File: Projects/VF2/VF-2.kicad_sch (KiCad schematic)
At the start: 16 parts, among them U1 OPA2134, U3 OPA2134

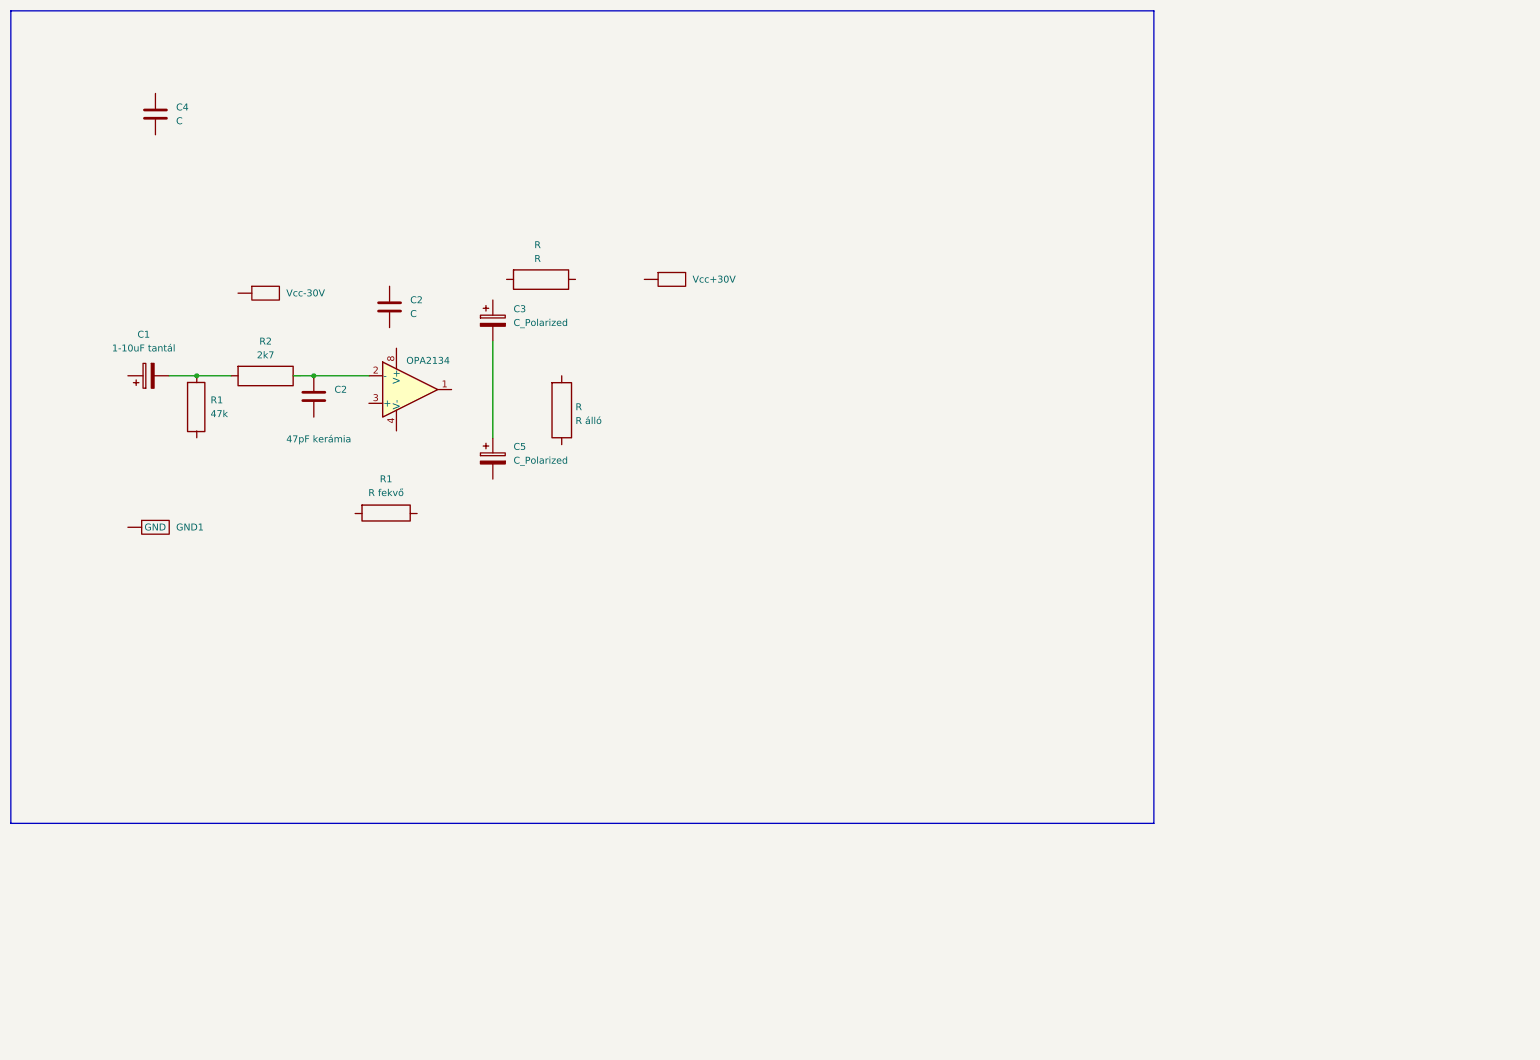
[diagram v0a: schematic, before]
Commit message: 1
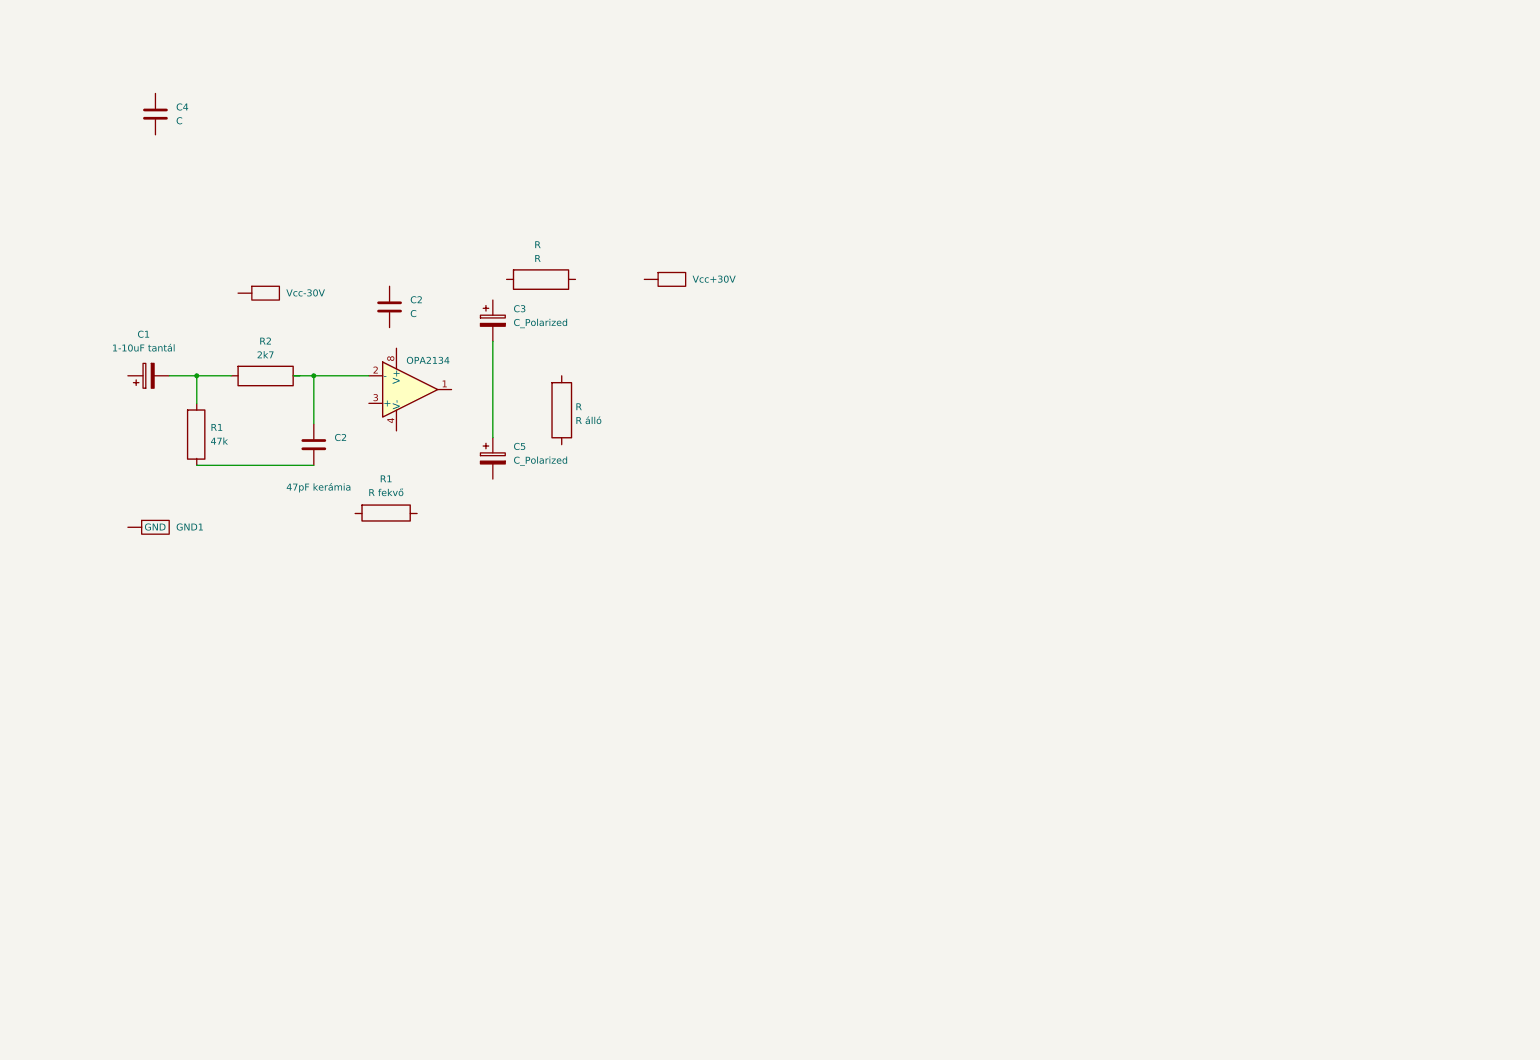
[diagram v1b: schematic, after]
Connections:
- net at C2.2: now also R1.1
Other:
- moved on the sheet: C2, R1
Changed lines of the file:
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@@
 	(generator_version "10.0")
 	(paper "A4")
-	(text_box ""
-		(exclude_from_sim no)
-		(at 0 0 0)
-		(size 210.82 149.86)
-		(margins 0.9525 0.9525 0.9525 0.9525)
-		(stroke
-			(width 0)
-			(type solid)
-		)
-		(fill
-			(type none)
-		)
-		(effects
-			(font
-				(size 1.27 1.27)
-			)
-			(justify left top)
-		)
+	(junction
+		(at 34.29 67.31)
+		(diameter 0)
+		(color 0 0 0 0)
 	)
 	(junction
@@
 		(color 0 0 0 0)
 	)
-	(junction
-		(at 34.29 67.31)
-		(diameter 0)
-		(color 0 0 0 0)
-	)
 	(wire
 		(pts
@@
 	(wire
 		(pts
-			(xy 29.21 67.31) (xy 34.29 67.31)
+			(xy 34.29 67.31) (xy 40.64 67.31)
 		)
 		(stroke
@@
 	(wire
 		(pts
-			(xy 66.04 67.31) (xy 55.88 67.31)
+			(xy 55.88 67.31) (xy 55.88 76.2)
 		)
 		(stroke
@@
 	(wire
 		(pts
-			(xy 88.9 60.96) (xy 88.9 78.74)
+			(xy 29.21 67.31) (xy 34.29 67.31)
 		)
 		(stroke
@@
 	(wire
 		(pts
-			(xy 34.29 67.31) (xy 40.64 67.31)
+			(xy 88.9 60.96) (xy 88.9 78.74)
 		)
 		(stroke
@@
 		)
 	)
+	(wire
+		(pts
+			(xy 34.29 72.39) (xy 34.29 67.31)
+		)
+		(stroke
+			(width 0)
+			(type default)
+		)
+	)
+	(wire
+		(pts
+			(xy 55.88 67.31) (xy 66.04 67.31)
+		)
+		(stroke
+			(width 0)
+			(type default)
+		)
+	)
+	(wire
+		(pts
+			(xy 34.29 83.82) (xy 55.88 83.82)
+		)
+		(stroke
+			(width 0)
+			(type default)
+		)
+	)
 	(symbol
 		(lib_id "Device:C")
@@
 	(symbol
 		(lib_id "Device:C")
-		(at 55.88 71.12 0)
+		(at 55.88 80.01 0)
 		(unit 1)
 		(body_style 1)
@@
 		(dnp no)
 		(property "Reference" "C2"
-			(at 59.69 69.8499 0)
+			(at 59.69 78.7399 0)
 			(show_name no)
 			(do_not_autoplace no)
@@
 		)
 		(property "Value" "47pF kerámia"
-			(at 50.8 78.994 0)
+			(at 50.8 87.884 0)
 			(show_name no)
 			(do_not_autoplace no)
@@
 		)
 		(property "Footprint" "Package_SO:SOIC-8_3.9x4.9mm_P1.27mm"
-			(at 56.8452 74.93 0)
-			(hide yes)
-			(show_name no)
-			(do_not_autoplace no)
-			(effects
-				(font
-					(size 1.27 1.27)
-				)
-			)
-		)
-		(property "Datasheet" ""
-			(at 55.88 71.12 0)
+			(at 56.8452 83.82 0)
+			(hide yes)
+			(show_name no)
+			(do_not_autoplace no)
+			(effects
+				(font
+					(size 1.27 1.27)
+				)
+			)
+		)
+		(property "Datasheet" ""
+			(at 55.88 80.01 0)
 			(hide yes)
 			(show_name no)
@@
 		)
 		(property "Description" "Unpolarized capacitor"
-			(at 55.88 71.12 0)
+			(at 55.88 80.01 0)
 			(hide yes)
 			(show_name no)
@@
 		(lib_name "R_álló_1")
 		(lib_id "001_Resistor_user:R_álló")
-		(at 34.29 76.2 0)
+		(at 34.29 81.28 0)
 		(unit 1)
 		(body_style 1)
@@
 		(fields_autoplaced yes)
 		(property "Reference" "R1"
-			(at 36.83 71.7998 0)
+			(at 36.83 76.8798 0)
 			(show_name no)
 			(do_not_autoplace no)
@@
 		)
 		(property "Value" "47k"
-			(at 36.83 74.3398 0)
+			(at 36.83 79.4198 0)
 			(show_name no)
 			(do_not_autoplace no)
@@
 		)
 		(property "Footprint" ""
-			(at 32.512 76.2 90)
-			(hide yes)
-			(show_name no)
-			(do_not_autoplace no)
-			(effects
-				(font
-					(size 1.27 1.27)
-				)
-			)
-		)
-		(property "Datasheet" ""
-			(at 34.29 76.2 0)
+			(at 32.512 81.28 90)
+			(hide yes)
+			(show_name no)
+			(do_not_autoplace no)
+			(effects
+				(font
+					(size 1.27 1.27)
+				)
+			)
+		)
+		(property "Datasheet" ""
+			(at 34.29 81.28 0)
 			(hide yes)
 			(show_name no)
@@
 		)
 		(property "Description" "Resistor"
-			(at 36.195 70.485 90)
-			(hide yes)
-			(show_name no)
+			(at 36.195 75.565 90)
+			(hide yes)
+			(show_name no)

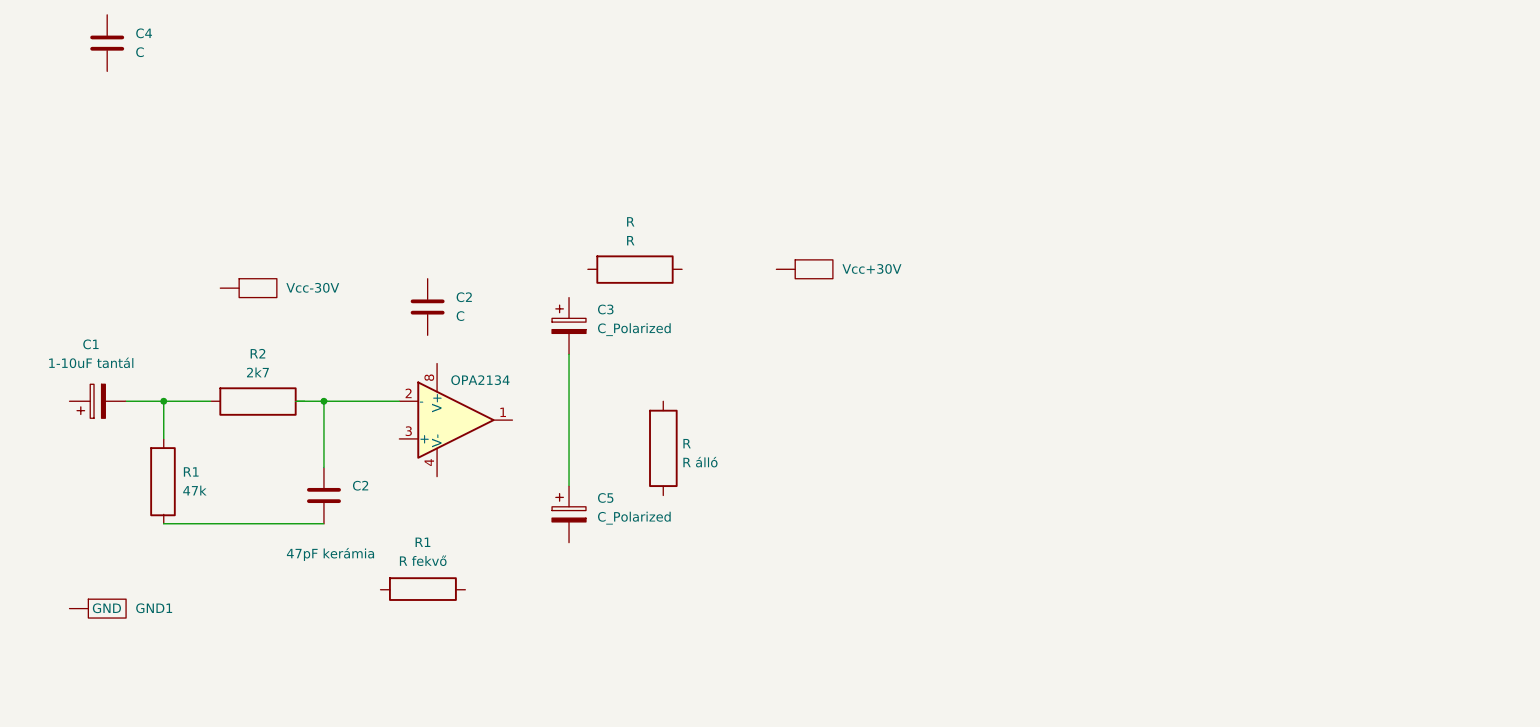
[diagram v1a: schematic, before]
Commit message: sch
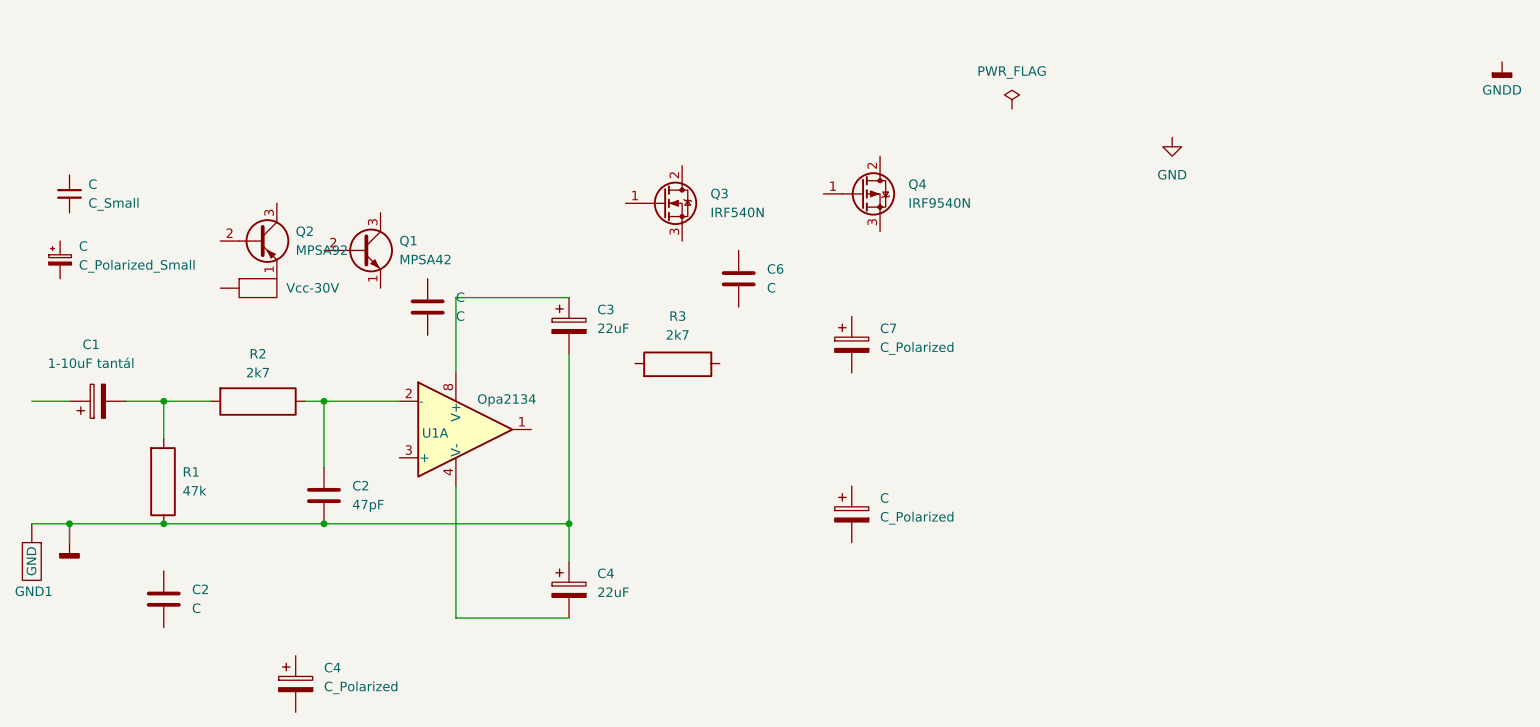
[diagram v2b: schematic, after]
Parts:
- removed C4: C, Package_SO:SOIC-8_3.9x4.9mm_P1.27mm, symbol Device:C
- removed R: R, symbol 001_Resistor_user:R
- removed R: R álló, symbol 001_Resistor_user:R_álló
- removed R1: R fekvő, symbol 001_Resistor_user:R
- removed U1: OPA2134, symbol Amplifier_Operational:OPA2134
- removed Vcc+30V: (no value), symbol 000_Device:Vcc
- added C: C_Polarized_Small, Package_SO:SOIC-8_3.9x4.9mm_P1.27mm, symbol Device:C_Polarized_Small
- added C: C_Small, symbol Device:C_Small
- added C, C4, C7: C_Polarized, Package_SO:SOIC-8_3.9x4.9mm_P1.27mm, symbol 000_Device:C_Polarized
- added C2, C6: C, Package_SO:SOIC-8_3.9x4.9mm_P1.27mm, symbol 000_Device:C
- added Q1: MPSA42, Package_TO_SOT_THT:TO-92_Inline, symbol Transistor_BJT:MPSA42
- added Q2: MPSA92, Package_TO_SOT_THT:TO-92_Inline, symbol Transistor_BJT:MPSA92
- added Q3: IRF540N, Package_TO_SOT_THT:TO-220-3_Vertical, symbol Transistor_FET:IRF540N
- added Q4: IRF9540N, Package_TO_SOT_THT:TO-220-3_Vertical, symbol Transistor_FET:IRF9540N
- added R3: 2k7, Package_SO:SOIC-8_3.9x4.9mm_P1.27mm, symbol 000_Device:R
- added U4: OPA2134, symbol 000_Device:OPA2134
- C2: value 47pF kerámia -> 47pF
- C3: value C_Polarized -> 22uF
- C4: renamed from C5; value C_Polarized -> 22uF
- U1: renamed from U3; value OPA2134 -> Opa2134
- renumbered C2 to C
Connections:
- net at R2.2: now also C2.1, U1.2 (-)
- net at C3.2, C4.1: now also C2.2, GND1. (GND), R1.1
- net at C4.2: now also U4.4 (V-)
- net at C3.1: now also U4.8 (V+)
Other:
- moved on the sheet: C4, GND1
